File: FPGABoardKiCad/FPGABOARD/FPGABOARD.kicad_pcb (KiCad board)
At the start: 4 copper layers, 78 x 51 mm, 80 parts, among them J1 USB_C_Receptacle_USB2.0_14P, J2 Program, J3 12PMOD, J4 6PMOD, J6 Conn_02x13_Odd_Even, SW1 ResetICE, SW2 BTN0, SW3 BTN1, SW4 BTN2, U1 AP2127K-1.2, U2 AP2127K-3.3, U3 W25Q32JVSS, U4 93LCxxBxxOT, U5 FT2232HPQ, U6 IS62LV256AL, U7 ICE40HX1K-VQ100, Y1 SG-210STF, Y2 SG-210STF

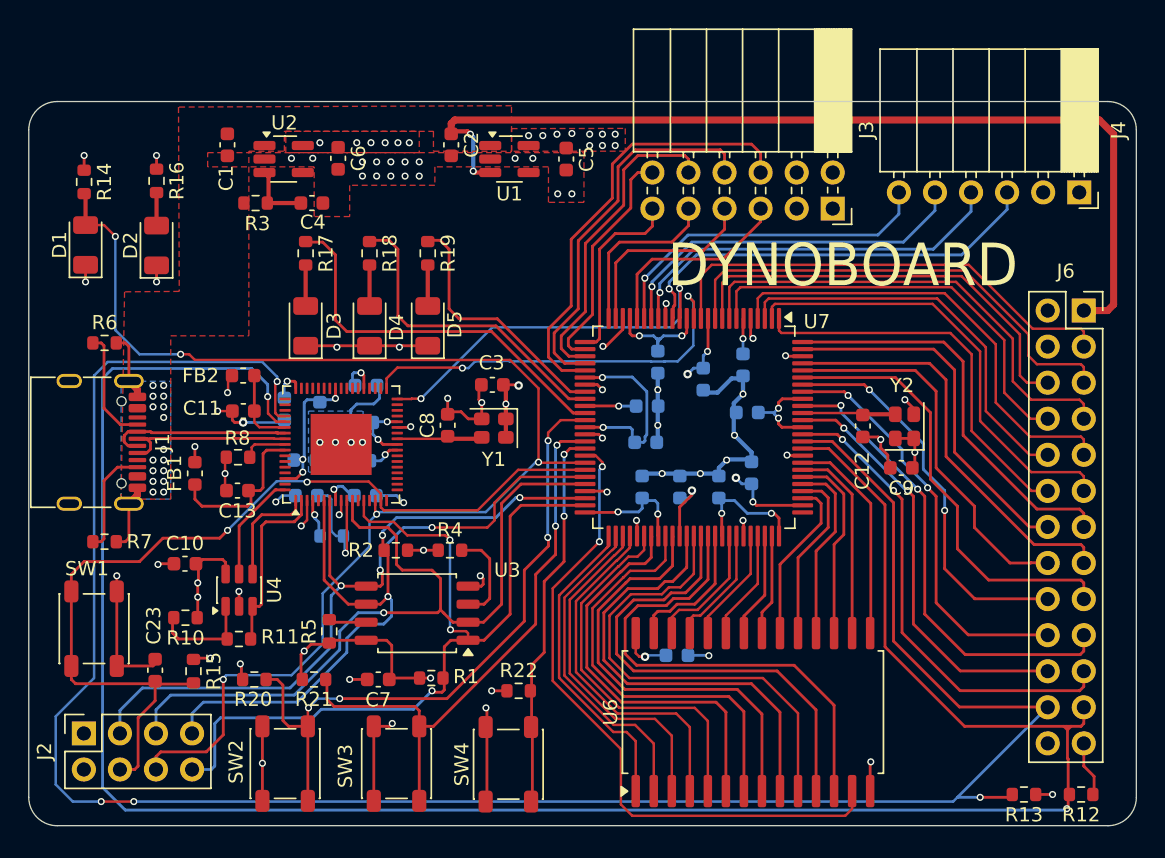
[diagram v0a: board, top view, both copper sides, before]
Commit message: Images
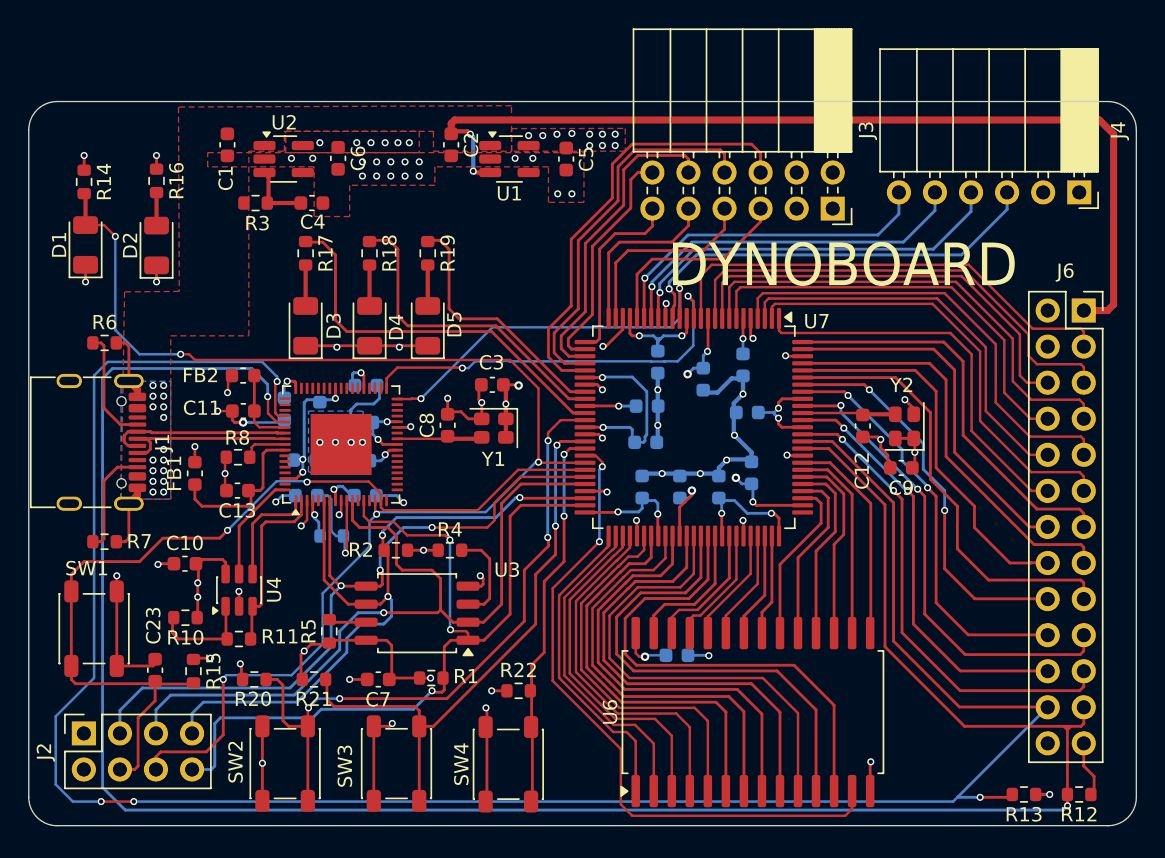
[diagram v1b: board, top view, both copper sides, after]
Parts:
- moved R12 0.14 mm to (154.0, 124.8)
